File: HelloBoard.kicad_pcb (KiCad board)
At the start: 2 copper layers, 38 parts, among them J1 USB_B_Micro, J2 Conn_01x04_Pin, J3 Conn_01x04_Pin, J4 Conn_02x08_Top_Bottom, SW1 SW_Push, SW2 SW_Push, U1 STM32F103C8T6, U2 AMS1117-3.3, U3 TMP235A2DCKR, U4 ADXL343, Y1 16MHz

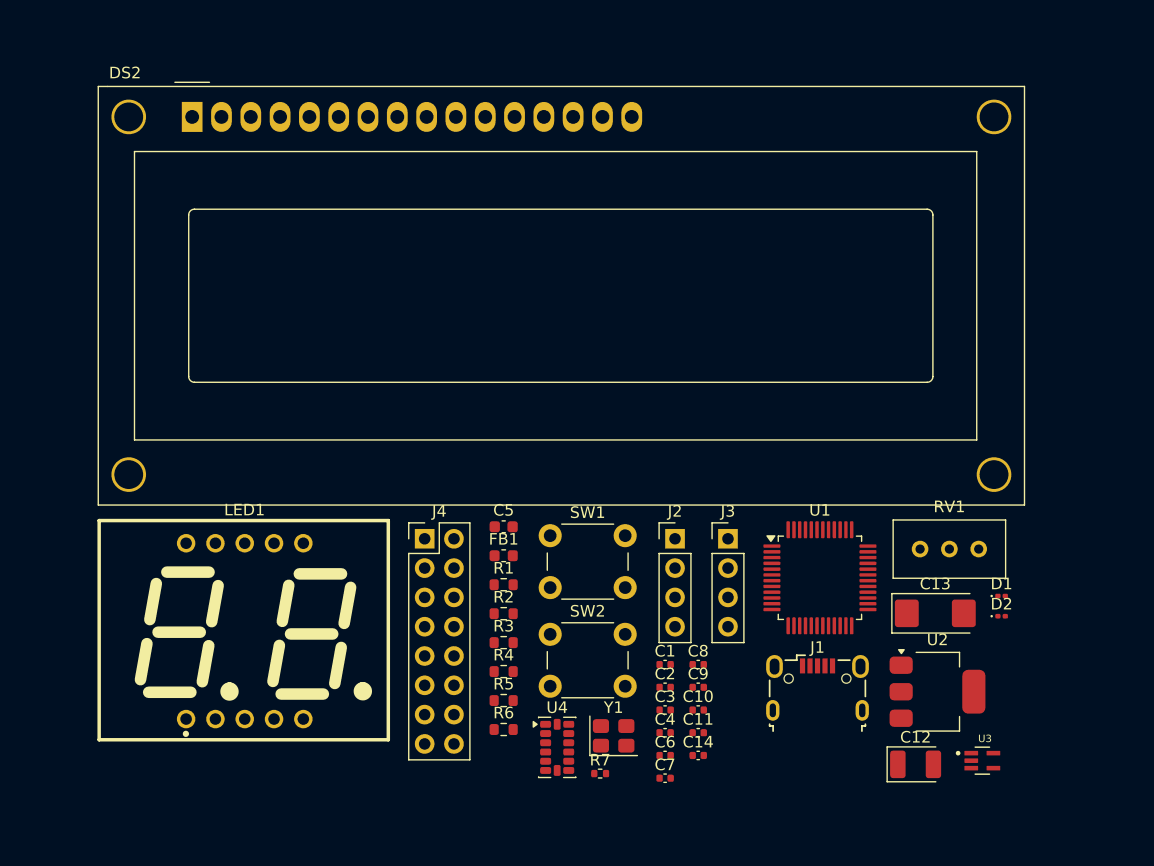
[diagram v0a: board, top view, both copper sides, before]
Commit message: started rough layout
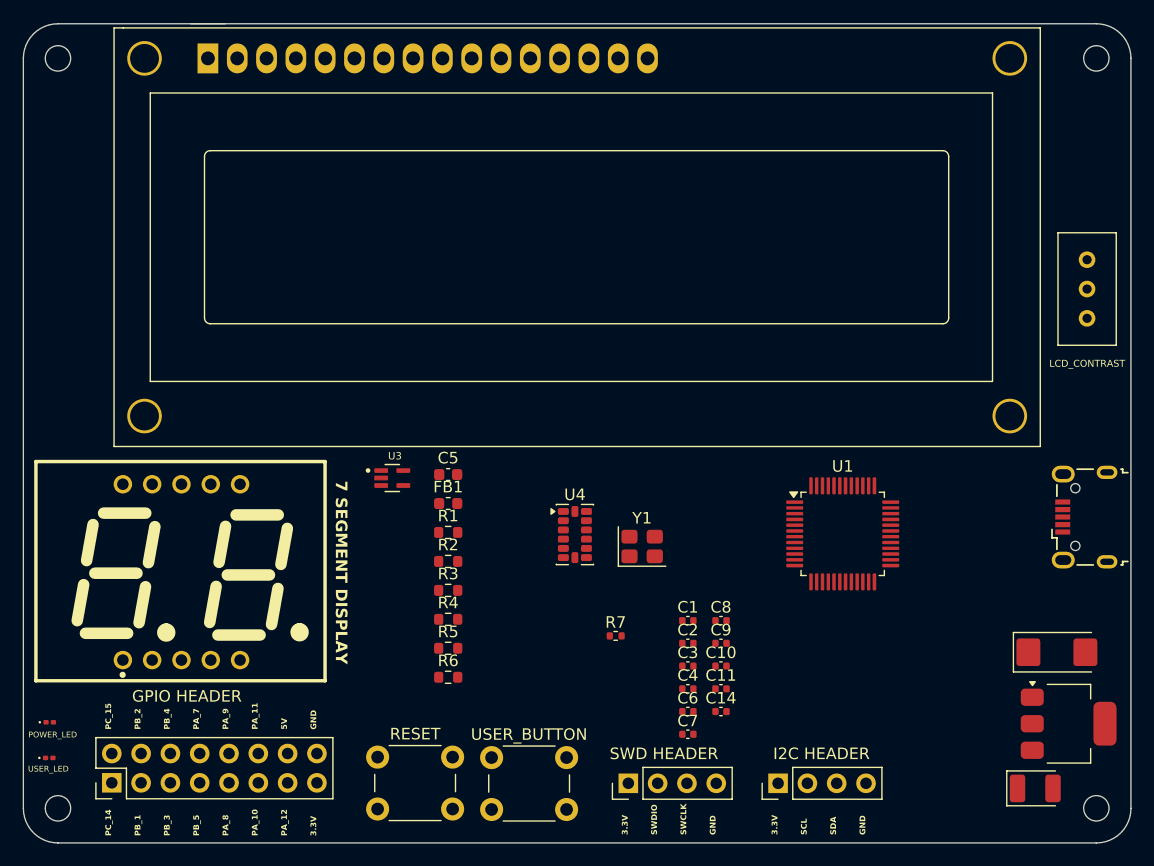
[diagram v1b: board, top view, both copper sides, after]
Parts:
- added H1: MountingHole, MountingHole:MountingHole_2.2mm_M2, F.Cu at (171.9, 24.7)
- added H2: MountingHole, MountingHole:MountingHole_2.2mm_M2, F.Cu at (81.9, 24.7)
- added H3: MountingHole, MountingHole:MountingHole_2.2mm_M2, F.Cu at (81.9, 89.7)
- added H4: MountingHole, MountingHole:MountingHole_2.2mm_M2, F.Cu at (171.9, 89.7)
- GPIO HEADER: renamed from J4
- I2C HEADER: renamed from J3
- SWD HEADER: renamed from J2
- USB CONNECTOR: renamed from J1
- moved USER_LED 83.5 mm to (81.2, 85.3)
- moved POWER_LED 83.2 mm to (81.2, 82.2)
- moved U3 56.7 mm to (110.9, 61.1)
- moved GPIO HEADER 34.4 mm to (86.6, 87.5), turned to 90 degrees
- moved USB CONNECTOR 27.5 mm to (170.9, 64.4), turned to 90 degrees
- moved LCD_CONTRAST 26.8 mm to (171.1, 42.1), turned to 90 degrees
- moved RESET 24.3 mm to (109.6, 85.2)
- moved I2C HEADER 21.6 mm to (144.3, 87.5), turned to 90 degrees
- moved SWD HEADER 21.6 mm to (131.3, 87.5), turned to 90 degrees
- moved U4 18.5 mm to (126.7, 66.0)
- moved Y1 16.6 mm to (132.5, 67.0)
- moved R7 12.0 mm to (130.3, 74.7)
- moved USER_BUTTON 11.8 mm to (119.5, 85.3)
- moved U2 11.7 mm to (169.5, 82.4)
- moved C13 11.1 mm to (168.5, 76.2)
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- renumbered RV1 to LCD_CONTRAST, D1 to POWER_LED, SW1 to RESET, SW2 to USER_BUTTON, D2 to USER_LED
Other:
- board outline added: 96 x 71 mm
- board text added: "3.3V"
- board text added: "5V"
- board text added: "7 SEGMENT DISPLAY"
- board text added: "GND"
- board text added: "PA_10"
- board text added: "PA_11"
- board text added: "PA_12"
- board text added: "PA_7"
- board text added: "PA_8"
- board text added: "PA_9"
- board text added: "PB_1"
- board text added: "PB_2"
- board text added: "PB_3"
- board text added: "PB_4"
- board text added: "PB_5"
- board text added: "PC_14"
- board text added: "PC_15"
- board text added: "SCL"
- board text added: "SDA"
- board text added: "SWCLK"
- board text added: "SWDIO"
